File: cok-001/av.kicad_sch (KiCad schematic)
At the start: 89 parts, among them J2401 AV OUT, Q2401 DTC144E, Q2402 SI2303BDS, Q2403 IMH20T108, Q2404 DTA144E, U2402 MC78M09, U2403 MC78M05, U2405 CX4351, U2409 LIGHT TRANSMITTER UNIT

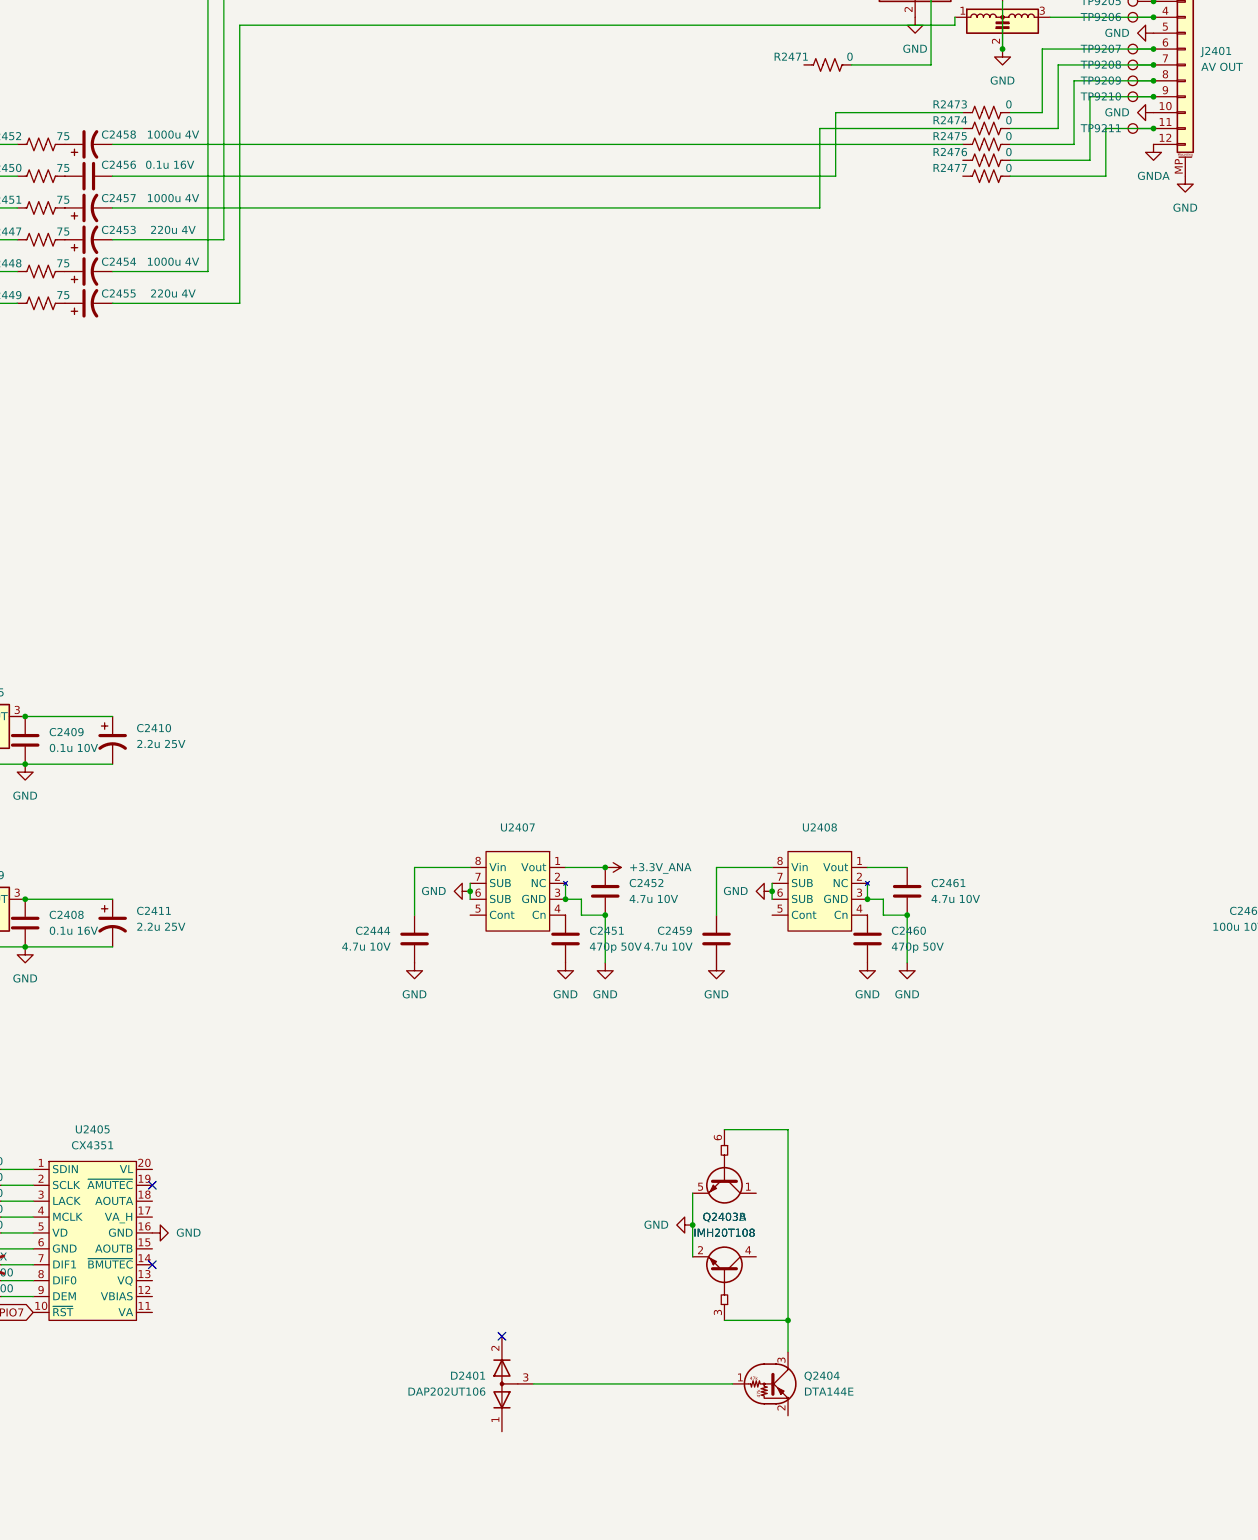
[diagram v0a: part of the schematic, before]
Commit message: voltage symbols
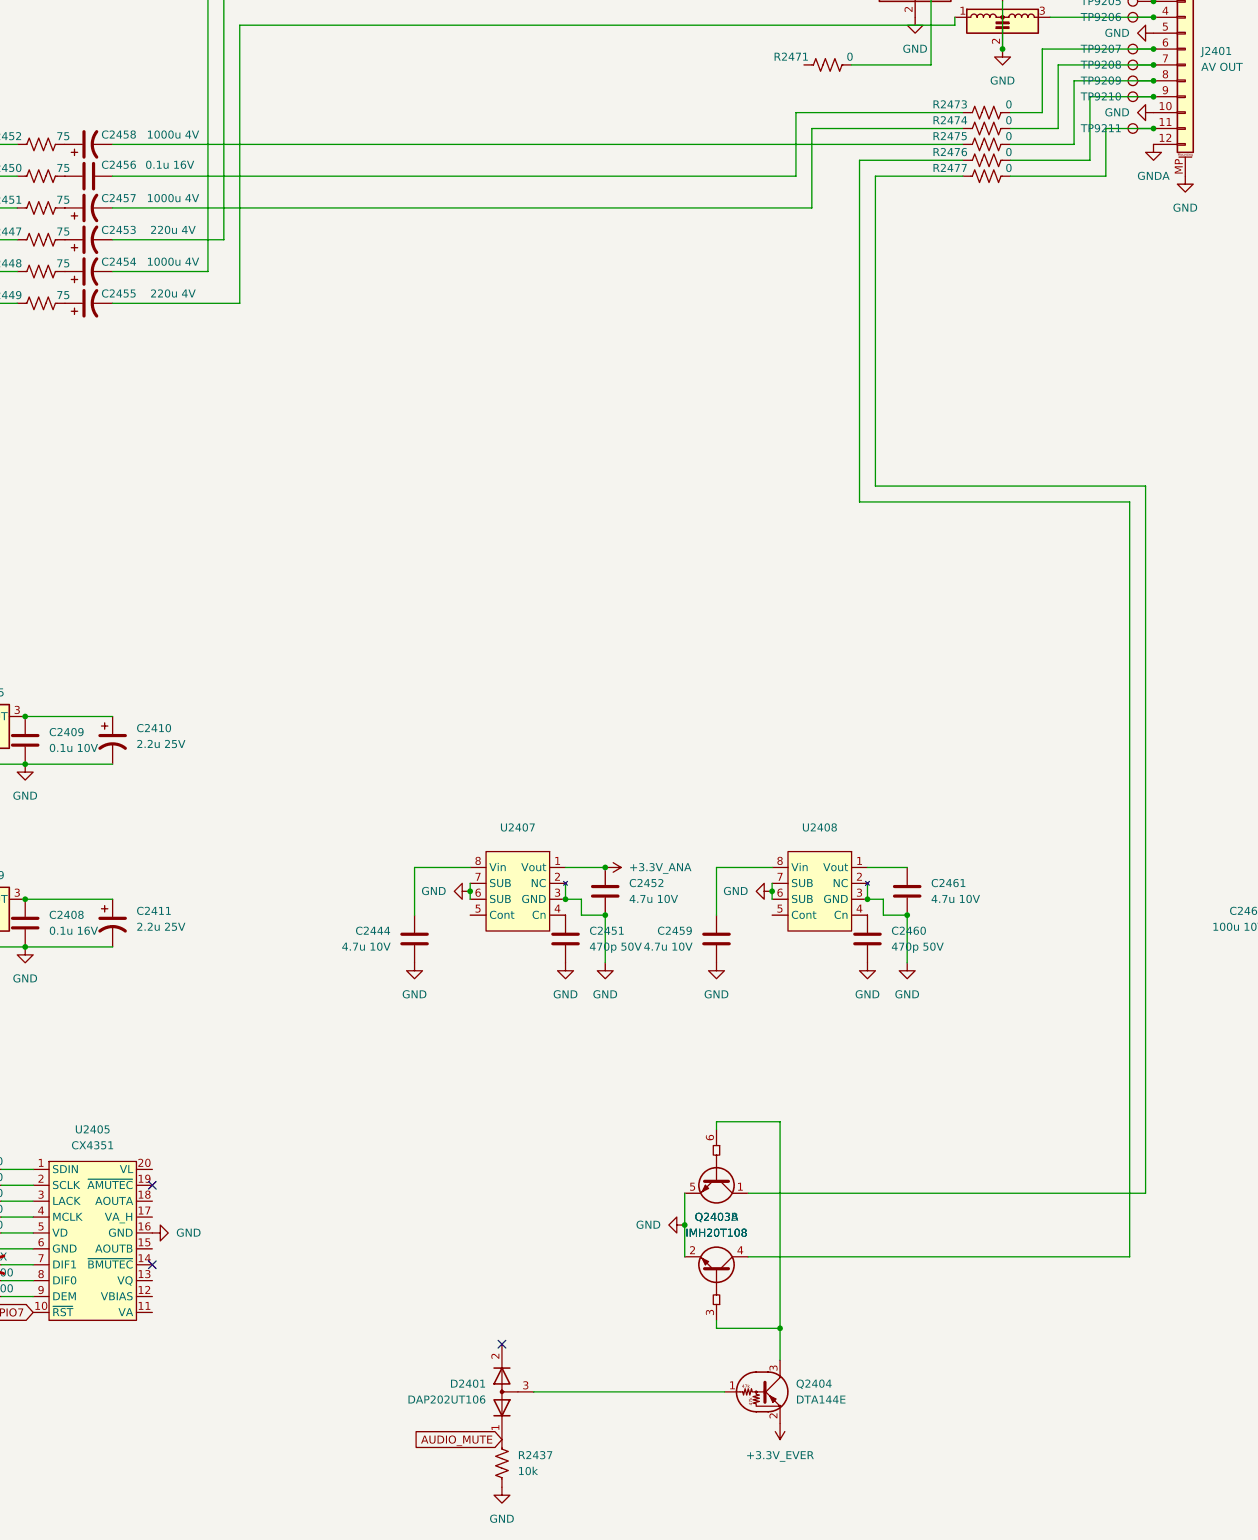
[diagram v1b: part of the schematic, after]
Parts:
- added R2437: 10k, Resistor_SMD:R_0402_1005Metric, symbol Device:R_US
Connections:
- net GND: now also R2437.1
- net +3.3V_EVER: now reaches Q2404.2 (E)
- net at Q2403.4 (C2): now also R2476.1
- net at R2477.1: now also Q2403.1 (C1)
- net AUDIO_MUTE: now reaches D2401.1 (K)
- net AUDIO_MUTE: now also R2437.2
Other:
- moved on the sheet: D2401, Q2403A, Q2403B, Q2404
